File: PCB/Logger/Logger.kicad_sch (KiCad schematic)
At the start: 73 parts, among them J2 USB-C-Socket-V, J3 JST-PH-SM4-TB, J3 USB-PROG, J5 Conn_01x05, J6 TF_PUSH, J8 Shelly, Q1 C179347, Q4 CJ2301, U1 TP4054, U10 ESP32-S3-MINI-1, U2 ME6211C33M5G-N

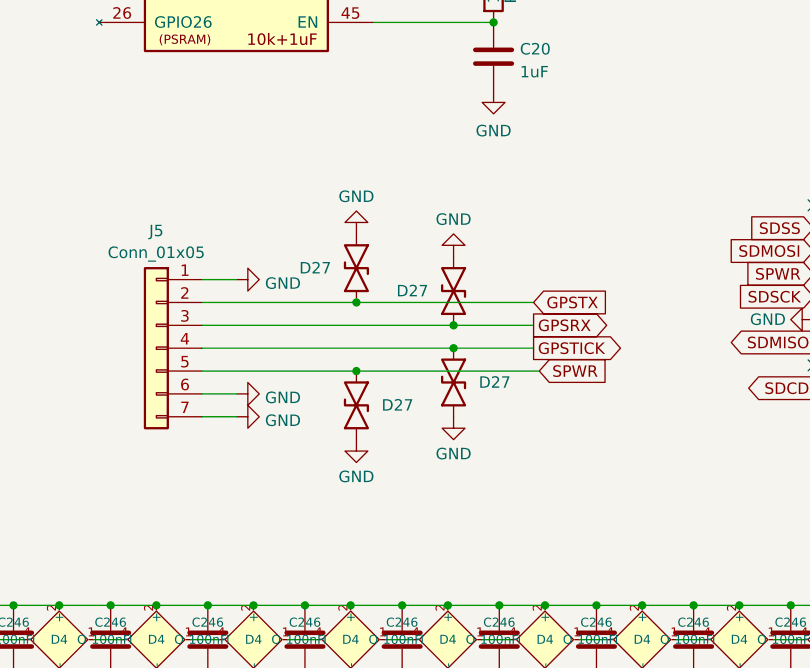
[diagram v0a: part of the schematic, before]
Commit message: ESD
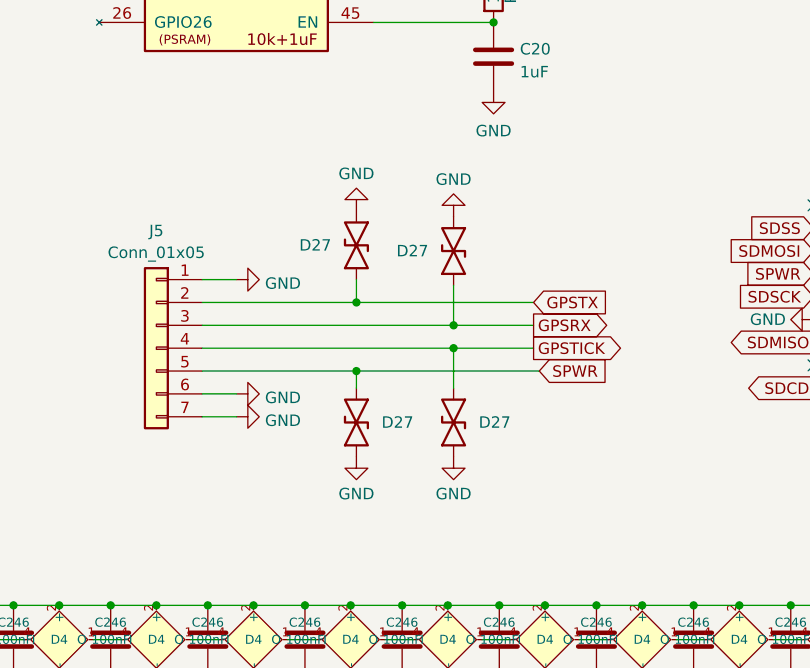
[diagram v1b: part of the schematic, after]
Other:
- moved on the sheet: D27
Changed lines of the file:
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@@
     (stroke (width 0) (type default))
   )
+  (wire (pts (xy 81.915 118.745) (xy 81.915 123.19))
+    (stroke (width 0) (type default))
+  )
   (wire (pts (xy 167.64 161.925) (xy 173.355 161.925))
     (stroke (width 0) (type default))
@@
     (stroke (width 0) (type default))
   )
+  (wire (pts (xy 81.915 130.175) (xy 81.915 125.73))
+    (stroke (width 0) (type default))
+  )
+  (wire (pts (xy 71.12 118.11) (xy 71.12 120.65))
+    (stroke (width 0) (type default))
+  )
   (wire (pts (xy 48.895 154.305) (xy 54.61 154.305))
     (stroke (width 0) (type default))
@@
     (stroke (width 0) (type default))
   )
+  (wire (pts (xy 71.12 130.175) (xy 71.12 128.27))
+    (stroke (width 0) (type default))
+  )
   (wire (pts (xy 81.28 154.305) (xy 86.995 154.305))
     (stroke (width 0) (type default))
@@
     )
   )
-  (symbol (lib_id "RevK:ES05D1MC10") (at 81.915 119.38 90) (unit 1)
+  (symbol (lib_id "RevK:ES05D1MC10") (at 81.915 114.935 90) (unit 1)
     (in_bom yes) (on_board yes) (dnp no)
-    (property "Reference" "D27" (at 75.565 119.38 90)
+    (property "Reference" "D27" (at 75.565 114.935 90)
       (effects (font (size 1.27 1.27)) (justify right))
     )
-    (property "Value" "~" (at 81.915 119.38 0)
+    (property "Value" "~" (at 81.915 114.935 0)
       (effects (font (size 1.27 1.27)))
     )
-    (property "Footprint" "RevK:DFN1006-2L" (at 78.74 118.745 0)
+    (property "Footprint" "RevK:DFN1006-2L" (at 78.74 114.3 0)
       (effects (font (size 1.27 1.27)) hide)
     )
-    (property "Datasheet" "" (at 81.915 119.38 0)
+    (property "Datasheet" "" (at 81.915 114.935 0)
       (effects (font (size 1.27 1.27)) hide)
     )
-    (property "LCSC Part #" "C5137770" (at 85.09 119.38 0)
+    (property "LCSC Part #" "C5137770" (at 85.09 114.935 0)
       (effects (font (size 1.27 1.27)) hide)
     )
@@
     )
   )
-  (symbol (lib_id "RevK:ES05D1MC10") (at 71.12 132.08 270) (unit 1)
+  (symbol (lib_id "RevK:ES05D1MC10") (at 71.12 133.985 270) (unit 1)
     (in_bom yes) (on_board yes) (dnp no)
-    (property "Reference" "D27" (at 77.47 132.08 90)
+    (property "Reference" "D27" (at 77.47 133.985 90)
       (effects (font (size 1.27 1.27)) (justify right))
     )
-    (property "Value" "~" (at 71.12 132.08 0)
+    (property "Value" "~" (at 71.12 133.985 0)
       (effects (font (size 1.27 1.27)))
     )
-    (property "Footprint" "RevK:DFN1006-2L" (at 74.295 132.715 0)
+    (property "Footprint" "RevK:DFN1006-2L" (at 74.295 134.62 0)
       (effects (font (size 1.27 1.27)) hide)
     )
-    (property "Datasheet" "" (at 71.12 132.08 0)
+    (property "Datasheet" "" (at 71.12 133.985 0)
       (effects (font (size 1.27 1.27)) hide)
     )
-    (property "LCSC Part #" "C5137770" (at 67.945 132.08 0)
+    (property "LCSC Part #" "C5137770" (at 67.945 133.985 0)
       (effects (font (size 1.27 1.27)) hide)
     )
@@
     )
   )
-  (symbol (lib_id "power:GND") (at 71.12 135.89 0) (unit 1)
+  (symbol (lib_id "power:GND") (at 71.12 137.795 0) (unit 1)
     (in_bom yes) (on_board yes) (dnp no) (fields_autoplaced)
-    (property "Reference" "#PWR0102" (at 71.12 142.24 0)
+    (property "Reference" "#PWR0102" (at 71.12 144.145 0)
       (effects (font (size 1.27 1.27)) hide)
     )
-    (property "Value" "GND" (at 71.12 140.0231 0)
+    (property "Value" "GND" (at 71.12 141.9281 0)
       (effects (font (size 1.27 1.27)))
     )
-    (property "Footprint" "" (at 71.12 135.89 0)
+    (property "Footprint" "" (at 71.12 137.795 0)
       (effects (font (size 1.27 1.27)) hide)
     )
-    (property "Datasheet" "" (at 71.12 135.89 0)
+    (property "Datasheet" "" (at 71.12 137.795 0)
       (effects (font (size 1.27 1.27)) hide)
     )
@@
     )
   )
-  (symbol (lib_id "power:GND") (at 81.915 115.57 180) (unit 1)
+  (symbol (lib_id "power:GND") (at 81.915 111.125 180) (unit 1)
     (in_bom yes) (on_board yes) (dnp no) (fields_autoplaced)
-    (property "Reference" "#PWR0102" (at 81.915 109.22 0)
+    (property "Reference" "#PWR0102" (at 81.915 104.775 0)
       (effects (font (size 1.27 1.27)) hide)
     )
-    (property "Value" "GND" (at 81.915 111.4369 0)
+    (property "Value" "GND" (at 81.915 106.9919 0)
       (effects (font (size 1.27 1.27)))
     )
-    (property "Footprint" "" (at 81.915 115.57 0)
+    (property "Footprint" "" (at 81.915 111.125 0)
       (effects (font (size 1.27 1.27)) hide)
     )
-    (property "Datasheet" "" (at 81.915 115.57 0)
+    (property "Datasheet" "" (at 81.915 111.125 0)
       (effects (font (size 1.27 1.27)) hide)
     )
@@
     )
   )
-  (symbol (lib_id "RevK:ES05D1MC10") (at 81.915 129.54 270) (unit 1)
+  (symbol (lib_id "RevK:ES05D1MC10") (at 81.915 133.985 270) (unit 1)
     (in_bom yes) (on_board yes) (dnp no)
-    (property "Reference" "D27" (at 88.265 129.54 90)
+    (property "Reference" "D27" (at 88.265 133.985 90)
       (effects (font (size 1.27 1.27)) (justify right))
     )
-    (property "Value" "~" (at 81.915 129.54 0)
+    (property "Value" "~" (at 81.915 133.985 0)
       (effects (font (size 1.27 1.27)))
     )
-    (property "Footprint" "RevK:DFN1006-2L" (at 85.09 130.175 0)
+    (property "Footprint" "RevK:DFN1006-2L" (at 85.09 134.62 0)
       (effects (font (size 1.27 1.27)) hide)
     )
-    (property "Datasheet" "" (at 81.915 129.54 0)
+    (property "Datasheet" "" (at 81.915 133.985 0)
       (effects (font (size 1.27 1.27)) hide)
     )
-    (property "LCSC Part #" "C5137770" (at 78.74 129.54 0)
+    (property "LCSC Part #" "C5137770" (at 78.74 133.985 0)
       (effects (font (size 1.27 1.27)) hide)
     )
@@
     )
   )
-  (symbol (lib_id "RevK:ES05D1MC10") (at 71.12 116.84 90) (unit 1)
+  (symbol (lib_id "RevK:ES05D1MC10") (at 71.12 114.3 90) (unit 1)
     (in_bom yes) (on_board yes) (dnp no)
-    (property "Reference" "D27" (at 64.77 116.84 90)
+    (property "Reference" "D27" (at 64.77 114.3 90)
       (effects (font (size 1.27 1.27)) (justify right))
     )
-    (property "Value" "~" (at 71.12 116.84 0)
+    (property "Value" "~" (at 71.12 114.3 0)
       (effects (font (size 1.27 1.27)))
     )
-    (property "Footprint" "RevK:DFN1006-2L" (at 67.945 116.205 0)
+    (property "Footprint" "RevK:DFN1006-2L" (at 67.945 113.665 0)
       (effects (font (size 1.27 1.27)) hide)
     )
-    (property "Datasheet" "" (at 71.12 116.84 0)
+    (property "Datasheet" "" (at 71.12 114.3 0)
       (effects (font (size 1.27 1.27)) hide)
     )
-    (property "LCSC Part #" "C5137770" (at 74.295 116.84 0)
+    (property "LCSC Part #" "C5137770" (at 74.295 114.3 0)
       (effects (font (size 1.27 1.27)) hide)
     )
@@
     )
   )
-  (symbol (lib_id "power:GND") (at 81.915 133.35 0) (unit 1)
+  (symbol (lib_id "power:GND") (at 81.915 137.795 0) (unit 1)
     (in_bom yes) (on_board yes) (dnp no) (fields_autoplaced)
-    (property "Reference" "#PWR0102" (at 81.915 139.7 0)
+    (property "Reference" "#PWR0102" (at 81.915 144.145 0)
       (effects (font (size 1.27 1.27)) hide)
     )
-    (property "Value" "GND" (at 81.915 137.4831 0)
+    (property "Value" "GND" (at 81.915 141.9281 0)
       (effects (font (size 1.27 1.27)))
     )
-    (property "Footprint" "" (at 81.915 133.35 0)
+    (property "Footprint" "" (at 81.915 137.795 0)
       (effects (font (size 1.27 1.27)) hide)
     )
-    (property "Datasheet" "" (at 81.915 133.35 0)
+    (property "Datasheet" "" (at 81.915 137.795 0)
       (effects (font (size 1.27 1.27)) hide)
     )
@@
     )
   )
-  (symbol (lib_id "power:GND") (at 71.12 113.03 180) (unit 1)
+  (symbol (lib_id "power:GND") (at 71.12 110.49 180) (unit 1)
     (in_bom yes) (on_board yes) (dnp no) (fields_autoplaced)
-    (property "Reference" "#PWR0102" (at 71.12 106.68 0)
+    (property "Reference" "#PWR0102" (at 71.12 104.14 0)
       (effects (font (size 1.27 1.27)) hide)
     )
-    (property "Value" "GND" (at 71.12 108.8969 0)
+    (property "Value" "GND" (at 71.12 106.3569 0)
       (effects (font (size 1.27 1.27)))
     )
-    (property "Footprint" "" (at 71.12 113.03 0)
+    (property "Footprint" "" (at 71.12 110.49 0)
       (effects (font (size 1.27 1.27)) hide)
     )
-    (property "Datasheet" "" (at 71.12 113.03 0)
+    (property "Datasheet" "" (at 71.12 110.49 0)
       (effects (font (size 1.27 1.27)) hide)
     )
